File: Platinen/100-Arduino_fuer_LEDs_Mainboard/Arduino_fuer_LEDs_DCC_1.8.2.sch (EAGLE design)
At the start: 115 parts, among them CON5 M04B4B-ZR4P, IC1 7805, IC2 LM393N, IC3 74125N, IC4 MCP2515-I/P, IC5 ISO1050, IC6 B0505S-1W, J1 day /night, J2 LocoNet, J3 SOLDERJUMPERNO, Q1 BC547, U1 WS2812_BREAKOUT, U2 LED NANO, U3 DCC NANO, U4 WS2812_BREAKOUT, X1 RJ10, X2 AK500/2+M, X3 MAB 5SH Conrad: 738247 - VQ, X4 AK500/2+M, X5 Reichelt MEBP 8-8S, X6 8 MHz, X7 AK500/2+M, X9 AK500/2+M

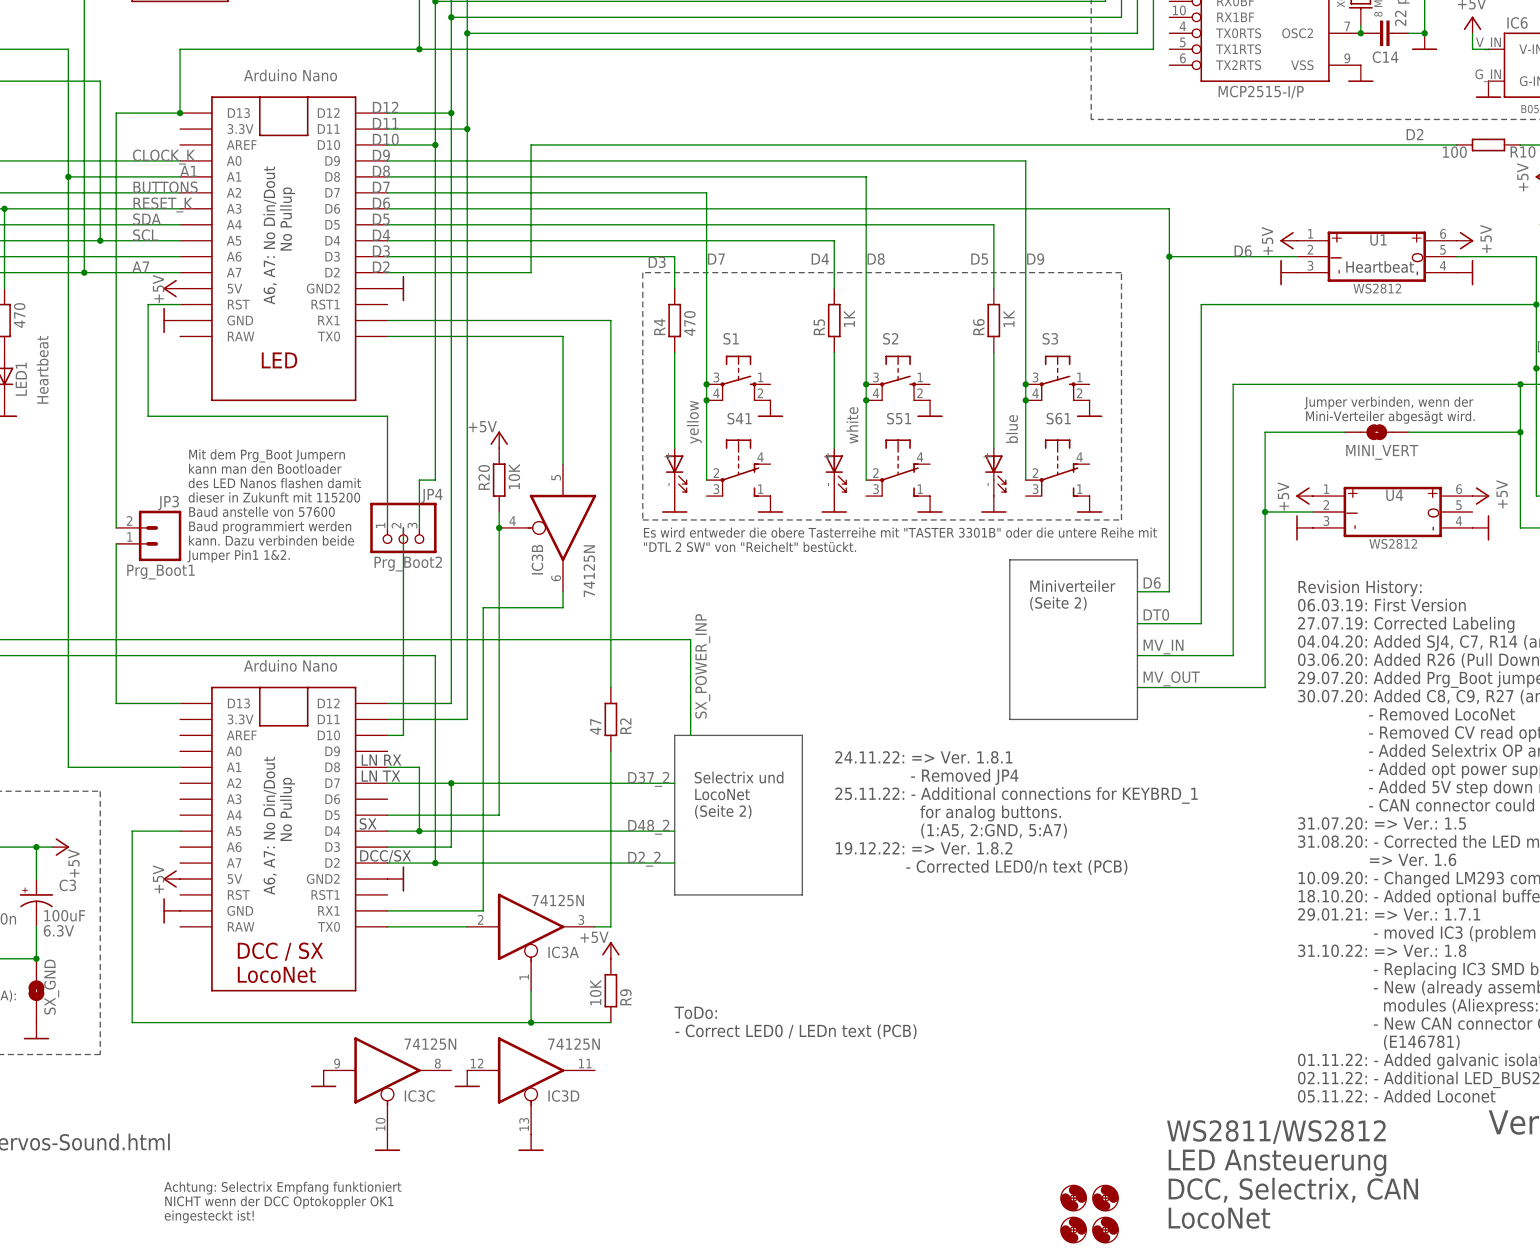
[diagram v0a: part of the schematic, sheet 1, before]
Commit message: Update Arduino_fuer_LEDs_DCC_1.8.2.sch
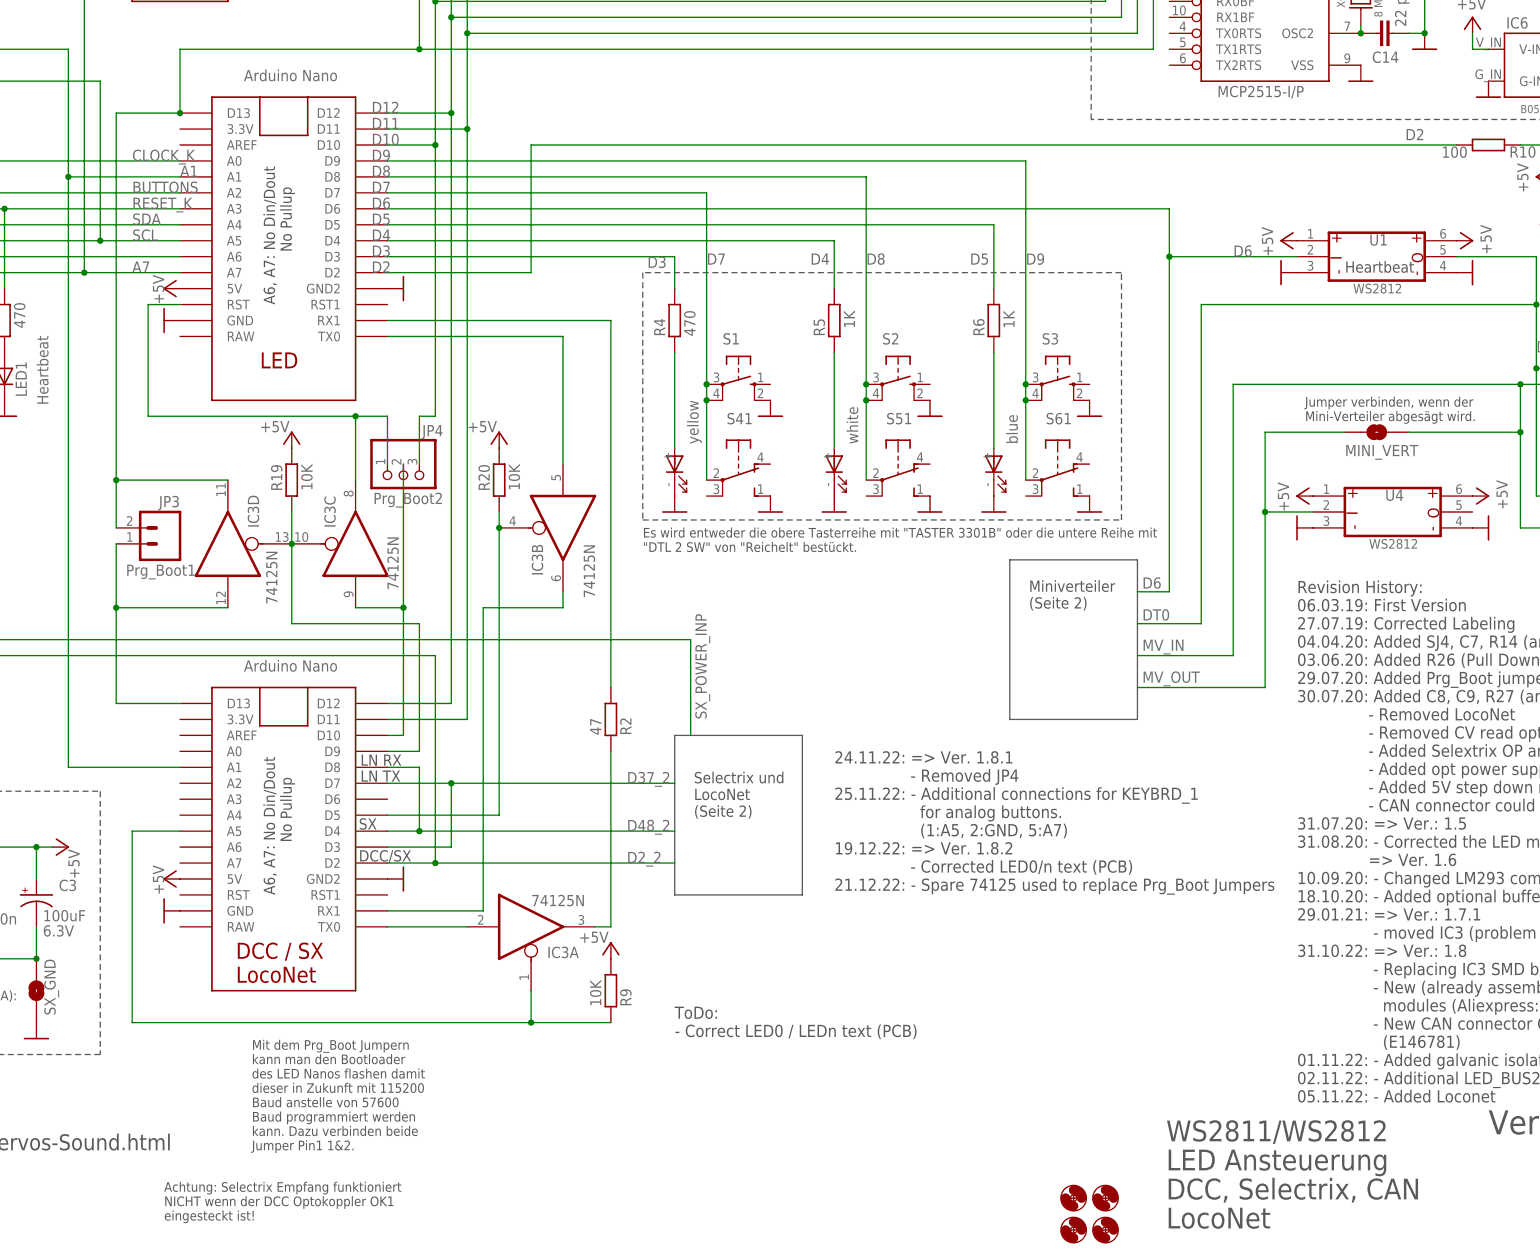
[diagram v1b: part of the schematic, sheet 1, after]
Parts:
- added R19: 10K, rcl:R-EU_0207/2V
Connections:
- new net N$11: IC3C.OE, IC3D.OE, R19.2, U3.D9
- net +5V: now also R19.1
- net D13: now also IC3D.O
- net GND: no longer IC3C.I, IC3C.OE, IC3D.I, IC3D.OE
- net N$15: now also IC3C.O
- net N$20: now also IC3D.I
- net N$28: now also IC3C.I
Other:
- note added: "24.11.22: => Ver. 1.8.1 - Removed JP4 25.11.22: - Additional connections for KEYBRD_1 for analog buttons. (1:A5, 2:GND, 5:A7) 19.12.22: => Ver. 1.8.2 - Corrected LED0/n text (PCB) 21.12.22: - Spare 74125 used to replace Prg_Boot Jumpers"
- note removed: "24.11.22: => Ver. 1.8.1 - Removed JP4 25.11.22: - Additional connections for KEYBRD_1 for analog buttons. (1:A5, 2:GND, 5:A7) 19.12.22: => Ver. 1.8.2 - Corrected LED0/n text (PCB)"
- moved on the sheet: IC3C, IC3D, JP4
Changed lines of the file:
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@@
 <part name="P+30" library="supply1" library_urn="urn:adsk.eagle:library:371" deviceset="+5V" device=""/>
 <part name="IC3" library="74xx-us" library_urn="urn:adsk.eagle:library:88" deviceset="74*125" device="N" package3d_urn="urn:adsk.eagle:package:16407/2"/>
-<part name="GND51" library="supply1" library_urn="urn:adsk.eagle:library:371" deviceset="GND" device=""/>
-<part name="GND52" library="supply1" library_urn="urn:adsk.eagle:library:371" deviceset="GND" device=""/>
-<part name="GND53" library="supply1" library_urn="urn:adsk.eagle:library:371" deviceset="GND" device=""/>
-<part name="GND54" library="supply1" library_urn="urn:adsk.eagle:library:371" deviceset="GND" device=""/>
 <part name="CON5" library="Connectors_Inline3_7" deviceset="M04" device="B4B-ZR4P" value="M04B4B-ZR4P"/>
 <part name="U1" library="Arduino_fuer_LEDs_DCC_2_All" deviceset="WS2812_BREAKOUT" device=""/>
@@
 <part name="SJ_SX6" library="SparkFun-Retired" deviceset="SOLDERJUMPER" device="NO"/>
 <part name="SJ_LN2" library="SparkFun-Retired" deviceset="SOLDERJUMPER" device="NO"/>
+<part name="R19" library="rcl" deviceset="R-EU_" device="0207/2V" value="10K"/>
+<part name="P+24" library="supply1" library_urn="urn:adsk.eagle:library:371" deviceset="+5V" device=""/>
 </parts>
 <sheets>
@@
 https://github.com/Hardi-St/MobaLedLib
 https://github.com/Hardi-St/MobaLedLib_Docu</text>
-<text x="31.75" y="81.28" size="1.524" layer="97">Mit dem Prg_Boot Jumpern
+<text x="41.91" y="-12.7" size="1.524" layer="97">Mit dem Prg_Boot Jumpern
 kann man den Bootloader
 des LED Nanos flashen damit
@@
                   (1:A5, 2:GND, 5:A7)
 19.12.22: =&gt; Ver. 1.8.2
-               - Corrected LED0/n text (PCB)</text>
+                - Corrected LED0/n text (PCB)
+21.12.22: - Spare 74125 used to replace Prg_Boot Jumpers</text>
 <text x="297.18" y="53.34" size="1.524" layer="97" align="top-left">Idee:
 - Zweite CS Leitung per Lötjumper damit man
@@
 <attribute name="NAME" x="30.48" y="89.662" size="1.778" layer="95" rot="MR0"/>
 </instance>
-<instance part="JP4" gate="A" x="66.04" y="83.82" smashed="yes" rot="MR270">
-<attribute name="NAME" x="72.39" y="90.805" size="1.778" layer="95" rot="MR0"/>
-<attribute name="VALUE" x="72.39" y="80.01" size="1.778" layer="96" rot="MR0"/>
+<instance part="JP4" gate="A" x="66.04" y="93.98" smashed="yes" rot="MR270">
+<attribute name="NAME" x="72.39" y="100.965" size="1.778" layer="95" rot="MR0"/>
+<attribute name="VALUE" x="72.39" y="90.17" size="1.778" layer="96" rot="MR0"/>
 </instance>
 <instance part="FRAME3" gate="G$1" x="-104.14" y="-30.48" smashed="yes">
@@
 <attribute name="VALUE" x="96.52" y="83.82" size="1.778" layer="96" rot="MR270"/>
 </instance>
-<instance part="IC3" gate="C" x="63.5" y="0" smashed="yes" rot="MR180">
-<attribute name="NAME" x="66.04" y="-3.175" size="1.778" layer="95" rot="MR180"/>
-<attribute name="VALUE" x="66.04" y="5.08" size="1.778" layer="96" rot="MR180"/>
-</instance>
-<instance part="IC3" gate="D" x="86.36" y="0" smashed="yes" rot="MR180">
-<attribute name="NAME" x="88.9" y="-3.175" size="1.778" layer="95" rot="MR180"/>
-<attribute name="VALUE" x="88.9" y="5.08" size="1.778" layer="96" rot="MR180"/>
-</instance>
-<instance part="GND51" gate="1" x="63.5" y="-12.7" smashed="yes"/>
-<instance part="GND52" gate="1" x="53.34" y="-2.54" smashed="yes"/>
-<instance part="GND53" gate="1" x="76.2" y="-2.54" smashed="yes"/>
-<instance part="GND54" gate="1" x="86.36" y="-12.7" smashed="yes"/>
+<instance part="IC3" gate="D" x="38.1" y="83.82" smashed="yes" rot="MR90">
+<attribute name="NAME" x="41.275" y="86.36" size="1.778" layer="95" rot="MR90"/>
+<attribute name="VALUE" x="44.196" y="74.168" size="1.778" layer="96" rot="MR90"/>
+</instance>
+<instance part="IC3" gate="C" x="58.42" y="83.82" smashed="yes" rot="R90">
+<attribute name="NAME" x="55.245" y="86.36" size="1.778" layer="95" rot="R90"/>
+<attribute name="VALUE" x="65.278" y="76.454" size="1.778" layer="96" rot="R90"/>
+</instance>
 <instance part="CON5" gate="G$1" x="147.32" y="213.36" smashed="yes" rot="MR270">
 <attribute name="VALUE" x="139.7" y="218.44" size="1.778" layer="96" rot="MR180"/>
@@
 <instance part="KEY_A7" gate="1" x="-20.32" y="127" smashed="yes" rot="R180">
 <attribute name="NAME" x="-15.24" y="125.73" size="1.778" layer="95" rot="R180"/>
+</instance>
+<instance part="R19" gate="G$1" x="48.26" y="93.98" smashed="yes" rot="MR270">
+<attribute name="NAME" x="46.7614" y="96.52" size="1.778" layer="95" rot="MR270"/>
+<attribute name="VALUE" x="51.562" y="96.52" size="1.778" layer="96" rot="MR270"/>
+</instance>
+<instance part="P+24" gate="1" x="48.26" y="101.6" smashed="yes">
+<attribute name="VALUE" x="43.18" y="101.6" size="1.778" layer="96"/>
 </instance>
 </instances>
@@
 </segment>
 <segment>
-<pinref part="IC3" gate="C" pin="OE"/>
-<pinref part="GND51" gate="1" pin="GND"/>
-</segment>
-<segment>
-<pinref part="IC3" gate="C" pin="I"/>
-<pinref part="GND52" gate="1" pin="GND"/>
-</segment>
-<segment>
-<pinref part="IC3" gate="D" pin="I"/>
-<pinref part="GND53" gate="1" pin="GND"/>
-</segment>
-<segment>
-<pinref part="IC3" gate="D" pin="OE"/>
-<pinref part="GND54" gate="1" pin="GND"/>
-</segment>
-<segment>
 <pinref part="U1" gate="G$1" pin="GND"/>
 <pinref part="GND6" gate="1" pin="GND"/>
@@
 <pinref part="P+35" gate="1" pin="+5V"/>
 </segment>
+<segment>
+<pinref part="R19" gate="G$1" pin="1"/>
+<pinref part="P+24" gate="1" pin="+5V"/>
+</segment>
 </net>
 <net name="D10" class="0">
@@
 <pinref part="CAN2" gate="1" pin="CS"/>
 <junction x="71.12" y="147.32"/>
-<wire x1="71.12" y1="93.98" x2="71.12" y2="147.32" width="0.1524" layer="91"/>
-<wire x1="68.58" y1="93.98" x2="71.12" y2="93.98" width="0.1524" layer="91"/>
+<wire x1="71.12" y1="104.14" x2="71.12" y2="147.32" width="0.1524" layer="91"/>
+<wire x1="68.58" y1="104.14" x2="71.12" y2="104.14" width="0.1524" layer="91"/>
 <pinref part="JP4" gate="A" pin="3"/>
-<wire x1="68.58" y1="86.36" x2="68.58" y2="93.98" width="0.1524" layer="91"/>
+<wire x1="68.58" y1="96.52" x2="68.58" y2="104.14" width="0.1524" layer="91"/>
 <wire x1="177.8" y1="170.18" x2="71.12" y2="170.18" width="0.1524" layer="91"/>
 <junction x="71.12" y="170.18"/>
@@
 <pinref part="U3" gate="G$1" pin="D13"/>
 <wire x1="30.48" y1="58.42" x2="20.32" y2="58.42" width="0.1524" layer="91"/>
-<wire x1="20.32" y1="58.42" x2="20.32" y2="83.82" width="0.1524" layer="91"/>
+<wire x1="20.32" y1="58.42" x2="20.32" y2="73.66" width="0.1524" layer="91"/>
 <pinref part="JP3" gate="G$1" pin="1"/>
+<pinref part="IC3" gate="D" pin="I"/>
+<wire x1="20.32" y1="73.66" x2="20.32" y2="83.82" width="0.1524" layer="91"/>
+<wire x1="38.1" y1="73.66" x2="20.32" y2="73.66" width="0.1524" layer="91"/>
+<junction x="20.32" y="73.66"/>
 </segment>
 </net>
@@
 <wire x1="66.04" y1="53.34" x2="63.5" y2="53.34" width="0.1524" layer="91"/>
 <pinref part="JP4" gate="A" pin="2"/>
-<wire x1="66.04" y1="86.36" x2="66.04" y2="53.34" width="0.1524" layer="91"/>
+<wire x1="66.04" y1="96.52" x2="66.04" y2="73.66" width="0.1524" layer="91"/>
+<pinref part="IC3" gate="C" pin="I"/>
+<wire x1="66.04" y1="73.66" x2="66.04" y2="53.34" width="0.1524" layer="91"/>
+<wire x1="58.42" y1="73.66" x2="66.04" y2="73.66" width="0.1524" layer="91"/>
+<junction x="66.04" y="73.66"/>
 </segment>
 </net>
@@
 <pinref part="U2" gate="G$1" pin="RST"/>
 <wire x1="25.4" y1="121.92" x2="30.48" y2="121.92" width="0.1524" layer="91"/>
-<wire x1="63.5" y1="104.14" x2="25.4" y2="104.14" width="0.1524" layer="91"/>
+<wire x1="63.5" y1="104.14" x2="58.42" y2="104.14" width="0.1524" layer="91"/>
 <pinref part="JP4" gate="A" pin="1"/>
-<wire x1="63.5" y1="104.14" x2="63.5" y2="86.36" width="0.1524" layer="91"/>
+<wire x1="58.42" y1="104.14" x2="25.4" y2="104.14" width="0.1524" layer="91"/>
+<wire x1="63.5" y1="104.14" x2="63.5" y2="96.52" width="0.1524" layer="91"/>
+<pinref part="IC3" gate="C" pin="O"/>
+<wire x1="58.42" y1="93.98" x2="58.42" y2="104.14" width="0.1524" layer="91"/>
+<junction x="58.42" y="104.14"/>
 </segment>
 </net>
@@
 <wire x1="78.74" y1="193.04" x2="68.58" y2="193.04" width="0.1524" layer="91"/>
 <pinref part="U2" gate="G$1" pin="D13"/>
-<wire x1="20.32" y1="86.36" x2="20.32" y2="152.4" width="0.1524" layer="91"/>
+<wire x1="20.32" y1="86.36" x2="20.32" y2="93.98" width="0.1524" layer="91"/>
+<wire x1="20.32" y1="93.98" x2="20.32" y2="152.4" width="0.1524" layer="91"/>
 <wire x1="30.48" y1="152.4" x2="20.32" y2="152.4" width="0.1524" layer="91"/>
 <pinref part="CAN2" gate="1" pin="CLK"/>
@@
 <wire x1="185.42" y1="162.56" x2="68.58" y2="162.56" width="0.1524" layer="91"/>
 <junction x="68.58" y="162.56"/>
+<pinref part="IC3" gate="D" pin="O"/>
+<wire x1="38.1" y1="93.98" x2="20.32" y2="93.98" width="0.1524" layer="91"/>
+<junction x="20.32" y="93.98"/>
 </segment>
 </net>
@@
 </segment>
 </net>
+<net name="N$11" class="0">
+<segment>
+<pinref part="IC3" gate="D" pin="OE"/>
+<pinref part="IC3" gate="C" pin="OE"/>
+<wire x1="48.26" y1="83.82" x2="48.26" y2="71.12" width="0.1524" layer="91"/>
+<junction x="48.26" y="83.82"/>
+<wire x1="48.26" y1="71.12" x2="68.58" y2="71.12" width="0.1524" layer="91"/>
+<wire x1="68.58" y1="71.12" x2="68.58" y2="50.8" width="0.1524" layer="91"/>
+<pinref part="U3" gate="G$1" pin="D9"/>
+<wire x1="68.58" y1="50.8" x2="63.5" y2="50.8" width="0.1524" layer="91"/>
+<pinref part="R19" gate="G$1" pin="2"/>
+<wire x1="48.26" y1="83.82" x2="48.26" y2="88.9" width="0.1524" layer="91"/>
+</segment>
+</net>
